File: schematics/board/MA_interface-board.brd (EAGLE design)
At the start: 39 x 26 mm, 30 parts

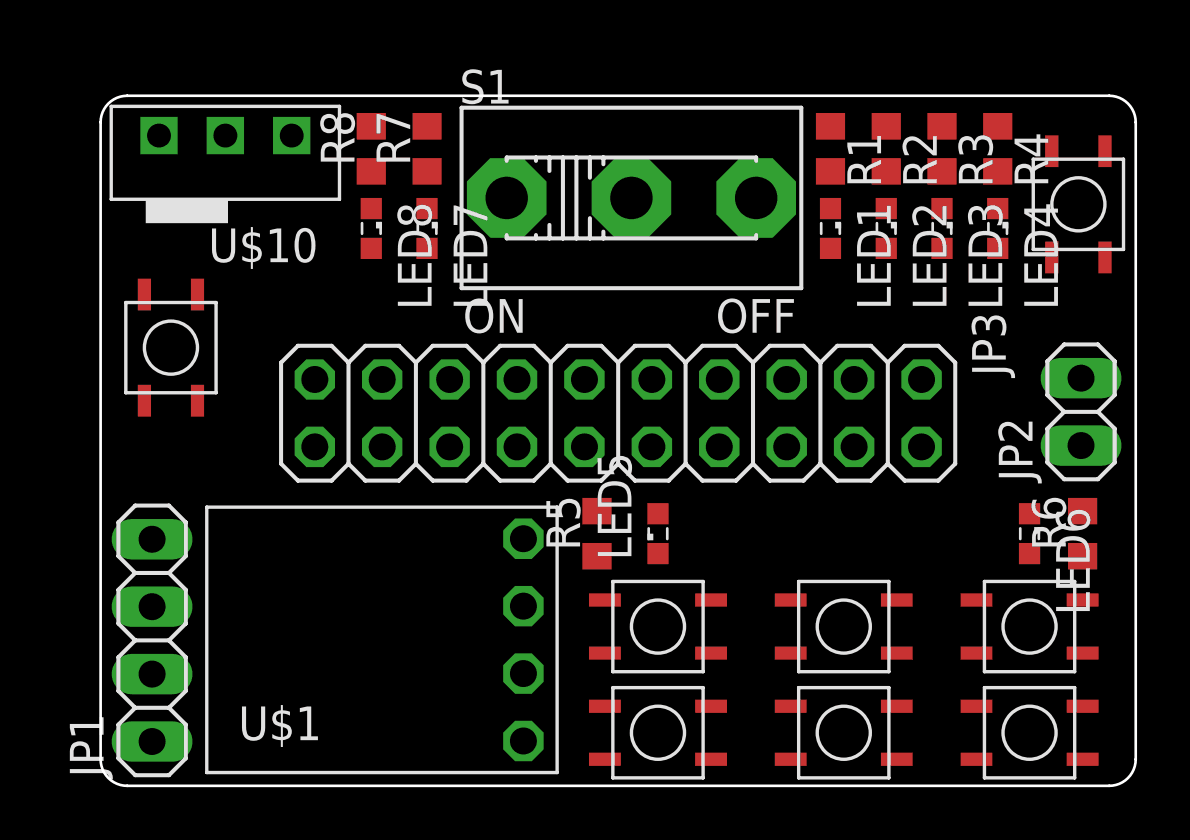
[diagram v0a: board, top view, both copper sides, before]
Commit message: Я Тимофей, и я сделал плату. Гыы...
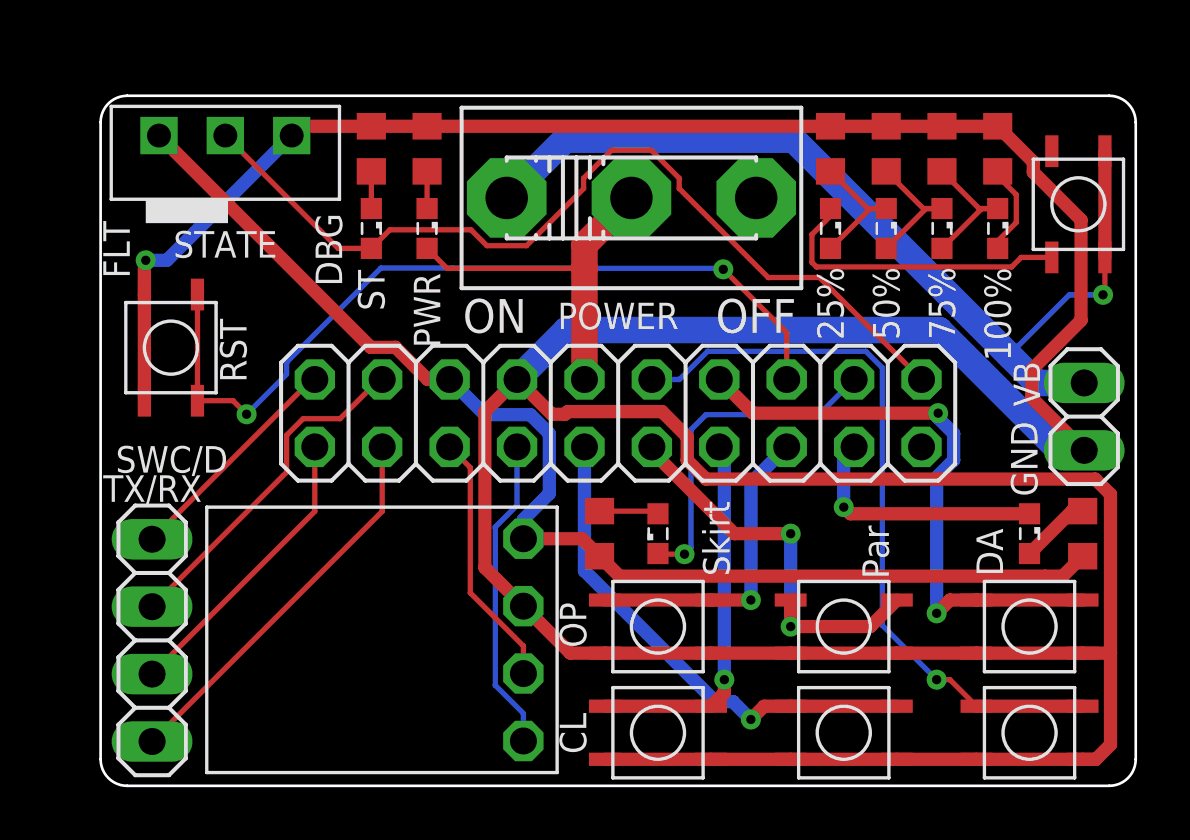
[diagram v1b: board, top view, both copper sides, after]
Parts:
- moved JP2 0.22 mm to (37.1, 13.9), turned to 270 degrees
- moved R5 0.10 mm to (18.8, 9.50), turned to 270 degrees
- turned R6 to 270 degrees
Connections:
- removed net DB_RX: JP1.1
- net DBG_RX: now also JP1.1
- net N$7: no longer U$2.P$4
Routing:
- net GND: track 0.00 -> 164.6 mm, vias 0 -> 1
- net 3V3: track 0.00 -> 45.7 mm
- net N$6: track 0.00 -> 36.4 mm, vias 0 -> 1
- net STATE: track 0.00 -> 34.1 mm
- net NRST: track 0.00 -> 31.7 mm, vias 0 -> 2
- net BOTTON_DA_DOWN: track 0.00 -> 27.9 mm, vias 0 -> 1
- net BOTTON_DA_UP: track 0.00 -> 22.5 mm, vias 0 -> 2
- net BOTTON_PAR_DOWN: track 0.00 -> 19.0 mm, vias 0 -> 1
- net BOTTON_PAR_UP: track 0.00 -> 15.6 mm, vias 0 -> 2
- net DBG_RX: track 0.00 -> 14.7 mm
- net BOTTON_SKIRT_CLOSE: track 0.00 -> 14.1 mm, vias 0 -> 1
- net V_BAT: track 0.00 -> 13.8 mm
- net SWD: track 0.00 -> 13.0 mm
- net FEEDBACK_SKIRT: track 0.00 -> 12.7 mm, vias 0 -> 1
- net SDA: track 0.00 -> 11.9 mm
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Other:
- board text added: "100%"
- board text added: "25%"
- board text added: "50%"
- board text added: "75%"
- board text added: "CL"
- board text added: "DA"
- board text added: "DBG"
- board text added: "FLT"
- board text added: "GND"
- board text added: "OP"
- board text added: "POWER"
- board text added: "PWR"
- board text added: "Par"
- board text added: "RST"
- board text added: "ST"
- board text added: "STATE"
- board text added: "SWC/D"
- board text added: "Skirt"
- board text added: "TX/RX"
- board text added: "VB"
